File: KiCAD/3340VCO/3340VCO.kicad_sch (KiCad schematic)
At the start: 74 parts, among them J1 ERK_PWR, J2 IN1, J3 IN2, J4 W_FORM, J5 TP_GND, J6 TP_GND, J7 OUT, SW1 SW_Rotary5, U1 NJM072D, U2 NJM072D, U3 NJM072D, U4 NJM072D, U5 AS3340

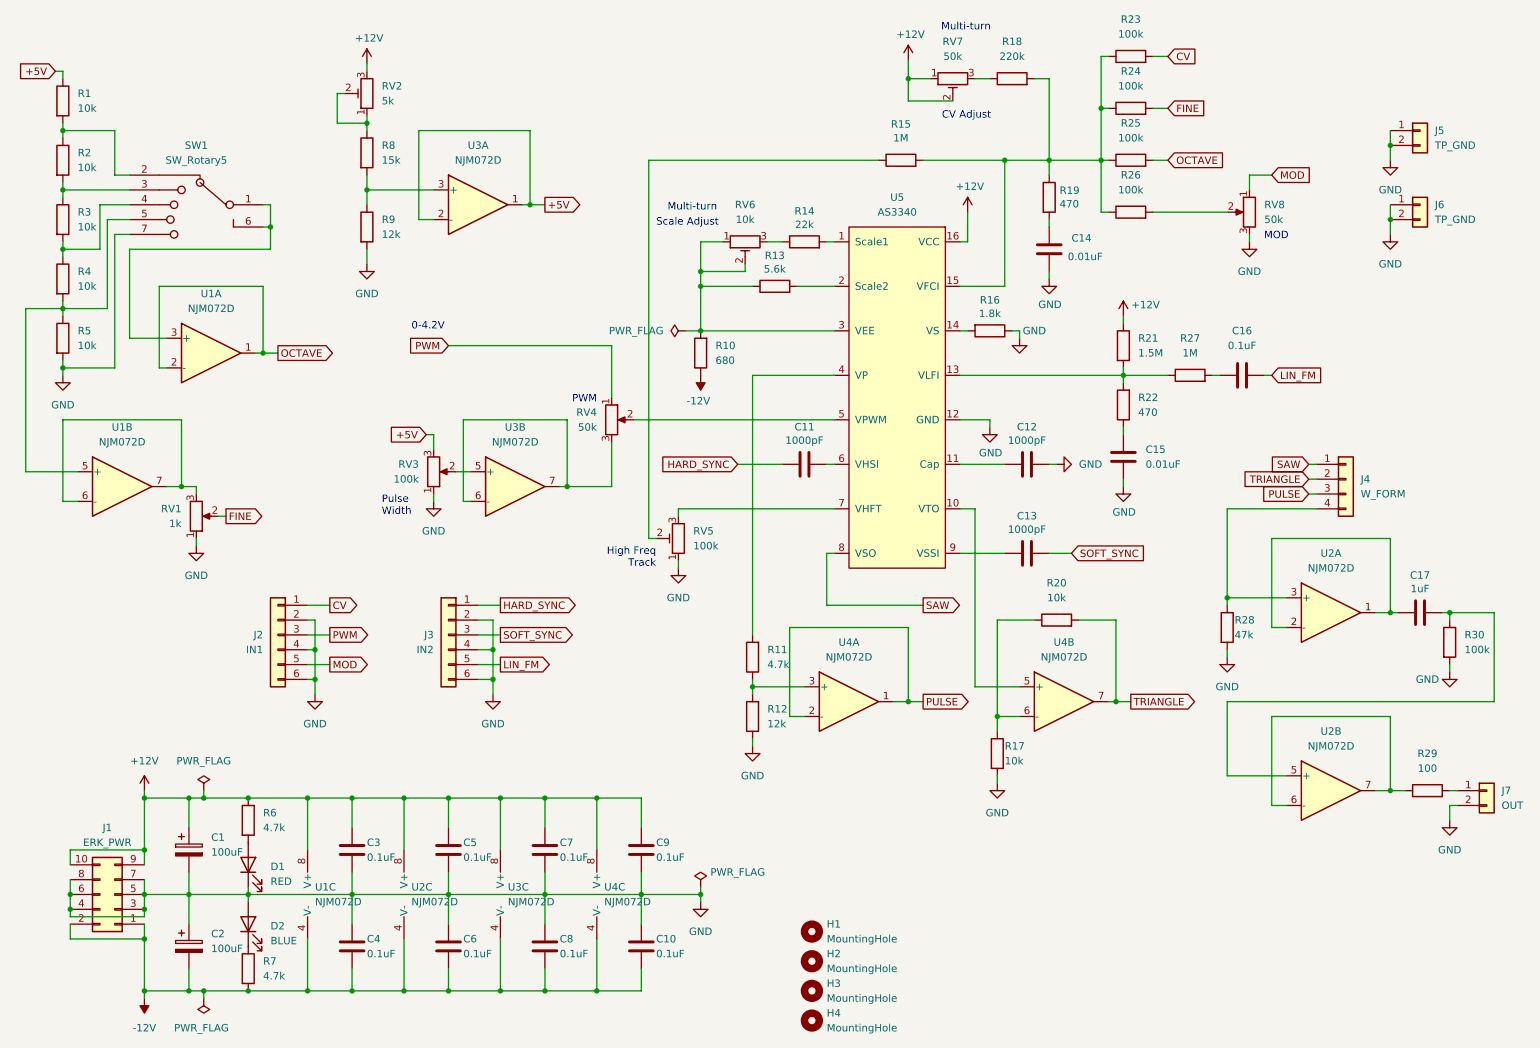
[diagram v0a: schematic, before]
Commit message: 部品配置
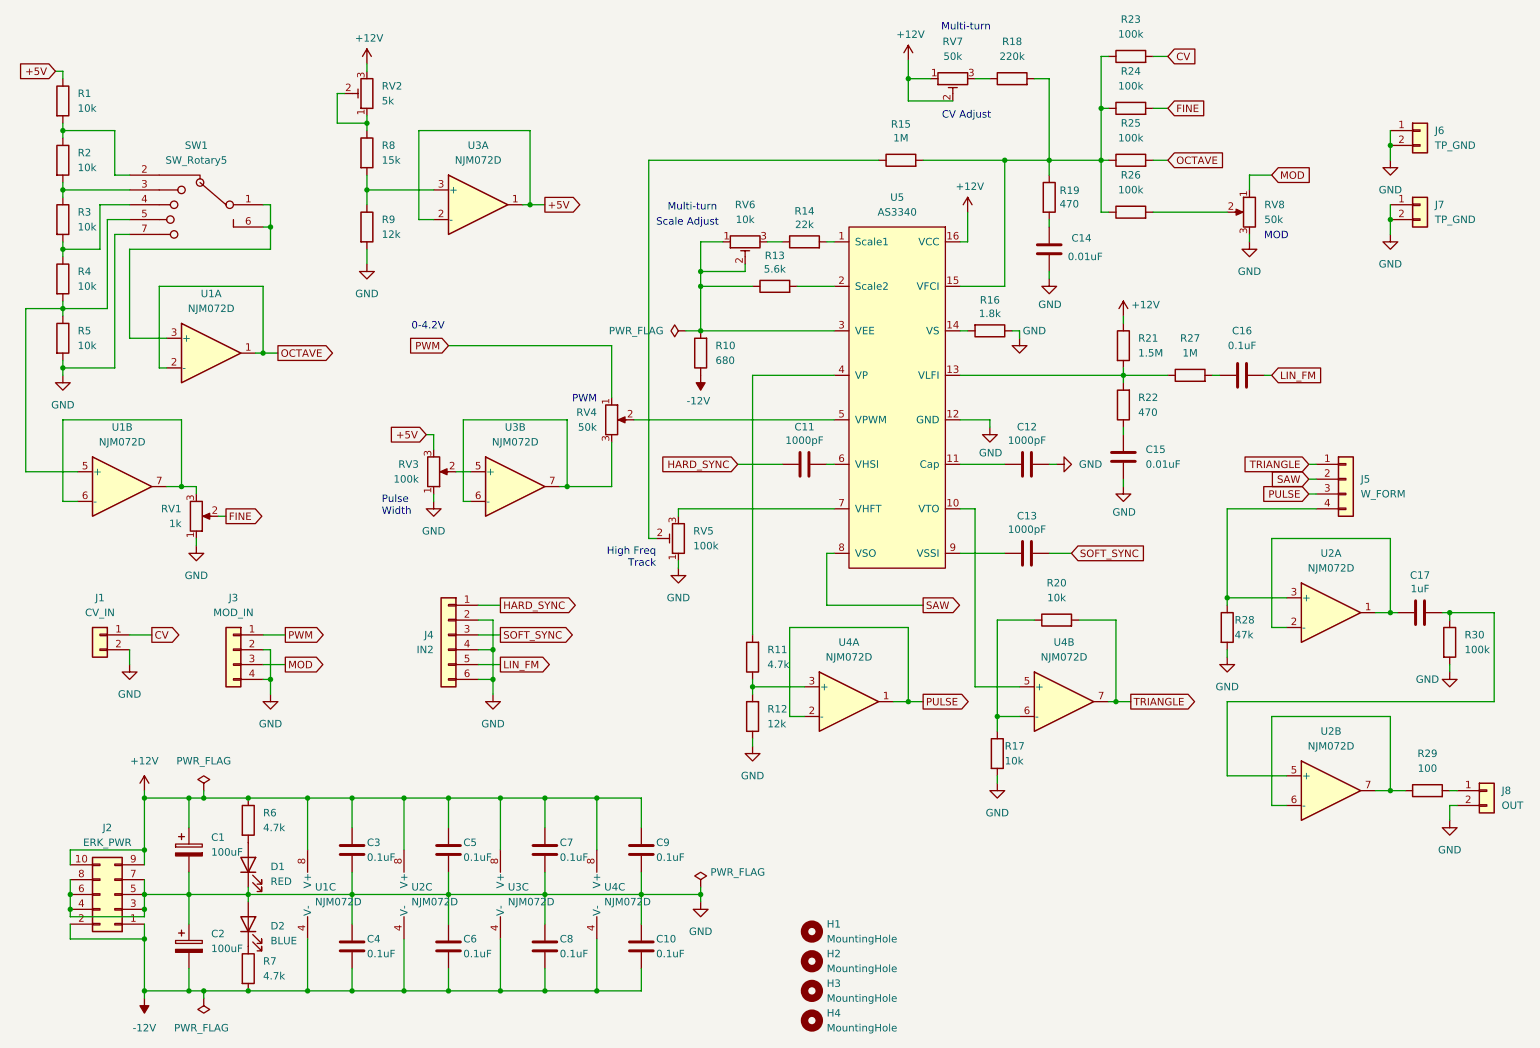
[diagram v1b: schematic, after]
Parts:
- removed J2: IN1, Connector_JST:JST_XH_B6B-XH-A_1x06_P2.50mm_Vertical, symbol Connector_Generic:Conn_01x06
- added J1: CV_IN, Connector_JST:JST_XH_B2B-XH-A_1x02_P2.50mm_Vertical, symbol Connector_Generic:Conn_01x02
- added J3: MOD_IN, Connector_JST:JST_XH_B4B-XH-A_1x04_P2.50mm_Vertical, symbol Connector_Generic:Conn_01x04
- renumbered J1 to J2, J3 to J4, J4 to J5, J5 to J6, J6 to J7, J7 to J8
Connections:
- net CV: now also J1.1 (Pin_1)
- net GND: now also J1.2 (Pin_2), J3.2 (Pin_2), J3.4 (Pin_4)
- net MOD: now also J3.3 (Pin_3)
- net PWM: now also J3.1 (Pin_1)
- net SAW: now also J5.2 (Pin_2); no longer J5.1 (Pin_1)
- net TRIANGLE: now also J5.1 (Pin_1); no longer J5.2 (Pin_2)
